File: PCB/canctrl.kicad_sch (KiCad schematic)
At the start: 18 parts, among them U4 SN65HVD230DR, U5 MCP2515-xSO, Y2 ABM8-16.000MHZ-B2-T

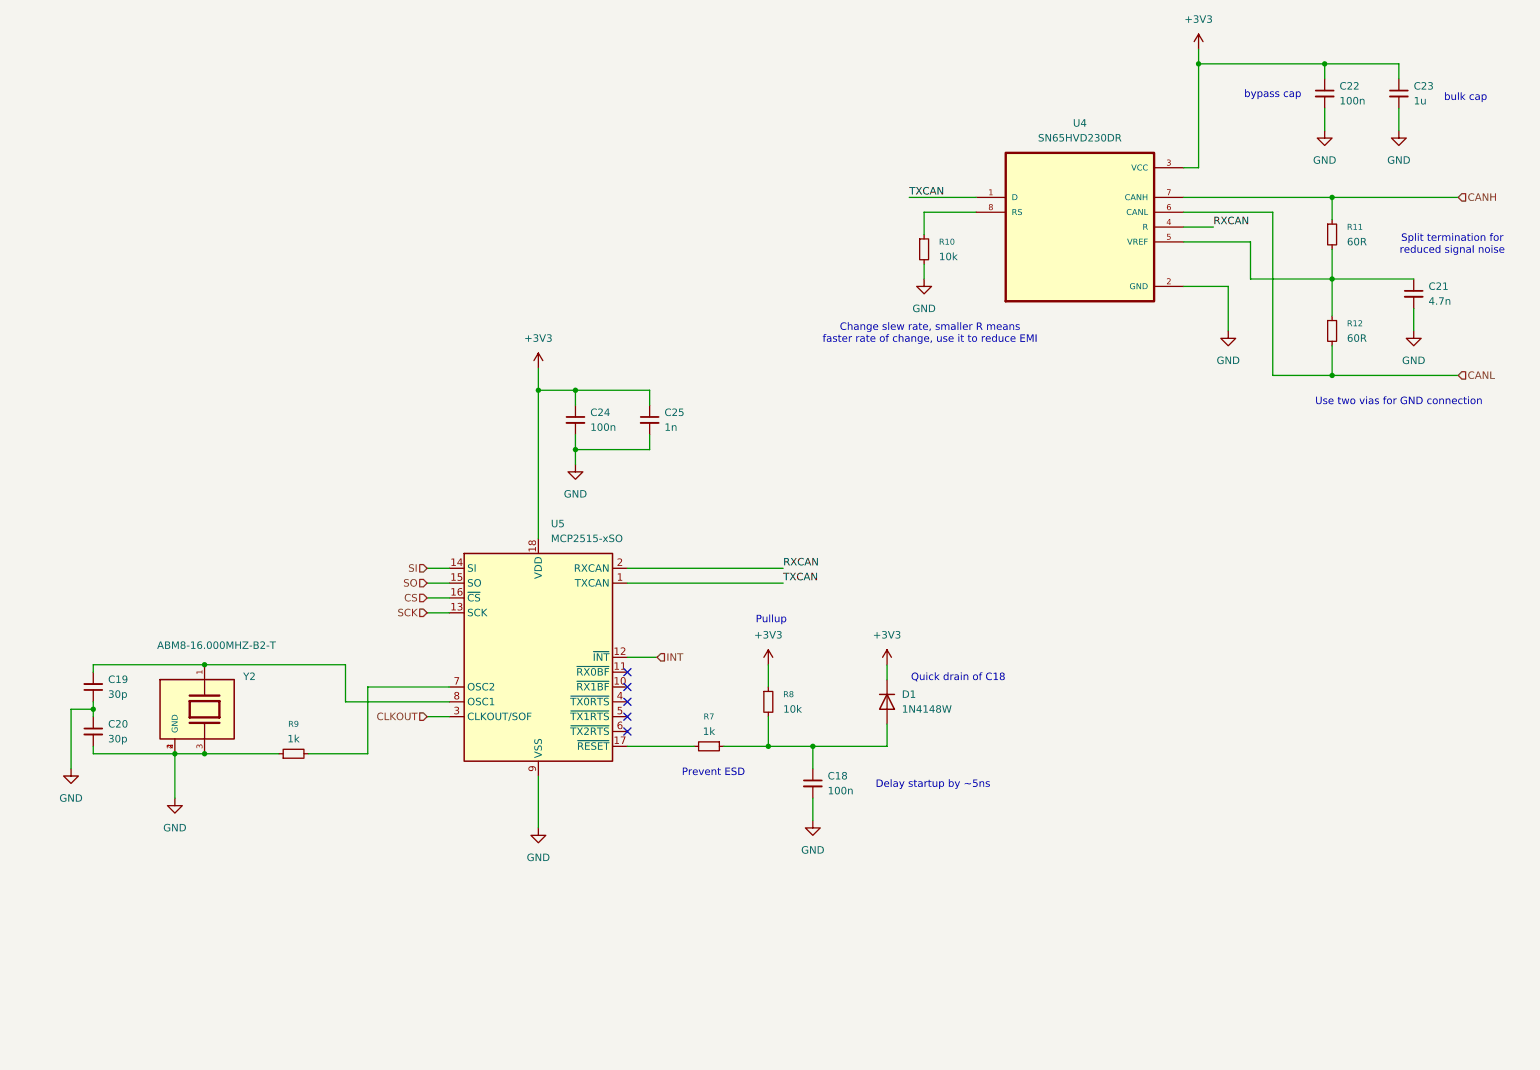
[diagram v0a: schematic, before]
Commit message: Routing PCB
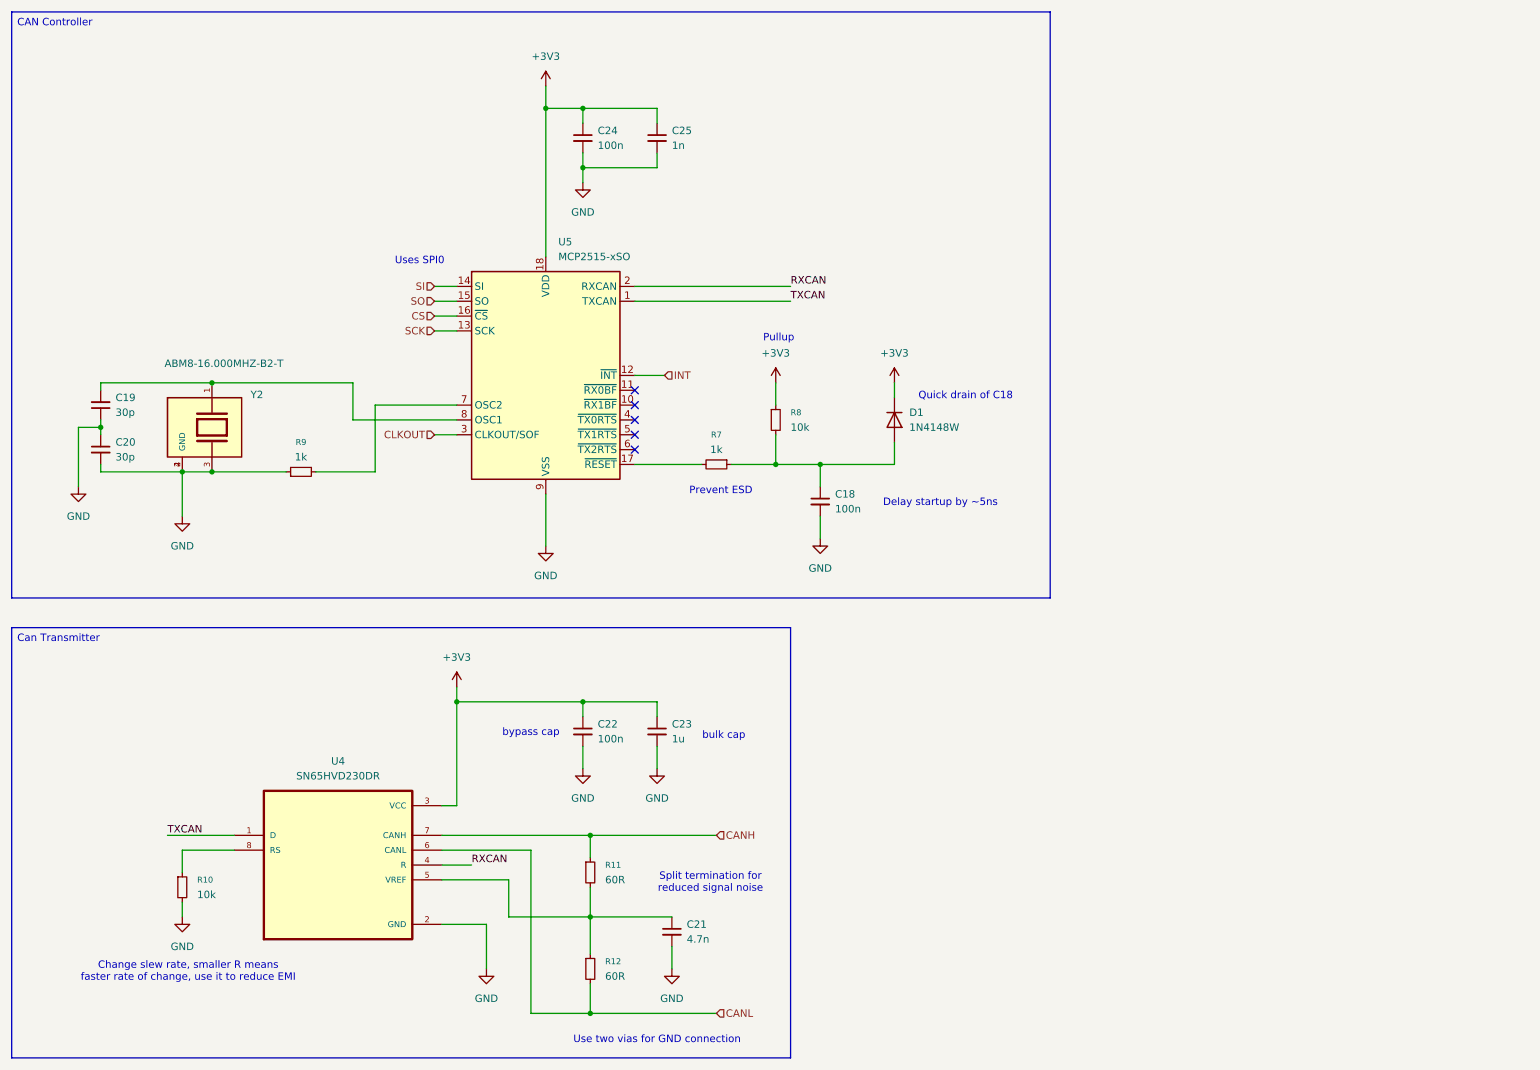
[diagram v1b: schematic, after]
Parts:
- C18, C19, C20, C21, C22, C23, C24, C25: footprint (none) -> Capacitor_SMD:C_0603_1608Metric_Pad1.08x0.95mm_HandSolder
- R10, R11, R12, R7, R8, R9: footprint (none) -> Resistor_SMD:R_0603_1608Metric_Pad0.98x0.95mm_HandSolder
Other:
- note added: "Uses SPI0"
- moved on the sheet: C18, C19, C20, C21, C22, C23, C24, C25, D1, R10, R11, R12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
